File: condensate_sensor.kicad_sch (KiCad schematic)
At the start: 3 parts

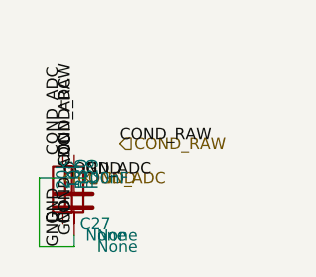
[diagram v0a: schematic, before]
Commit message: fic placer for small schemes
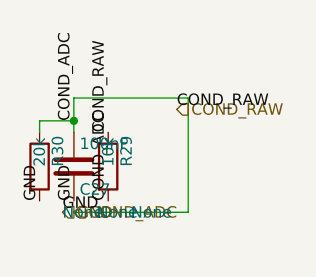
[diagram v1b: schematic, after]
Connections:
- net COND_ADC: no longer C27.2, R30.2
- new net GND: C27.2, R30.2
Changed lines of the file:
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@@
 	(symbol
 		(lib_id "Device:C")
-		(at 16.51 19.05 0)
+		(at 16.51 15.24 0)
 		(unit 1)
 		(exclude_from_sim no)
@@
 		(fields_autoplaced no)
 		(property "Reference" "C27"
-			(at 17.145 21.59 0.0000)
+			(at 17.145 17.78 0.0000)
 			(effects
 				(font
@@
 		)
 		(property "Value" "100nF"
-			(at 17.145 16.51 0.0000)
+			(at 17.145 12.7 0.0000)
 			(effects
 				(font
@@
 		)
 		(property "mirror" "None"
-			(at 19.05 24.1299 0)
+			(at 19.05 20.3199 0)
 			(effects
 				(font
@@
 		(instances
 			(project "Untitled"
-				(path "/aeae88a2-db2d-48e3-a72d-65ba09dff43f"
+				(path "/6ad2648c-8bf5-446b-ae62-81d18f8efea8"
 					(reference "C27")
 					(unit 1)
@@
 	(symbol
 		(lib_id "Device:R")
-		(at 16.51 17.78 0)
+		(at 20.32 15.24 0)
 		(unit 1)
 		(exclude_from_sim no)
@@
 		(fields_autoplaced no)
 		(property "Reference" "R29"
-			(at 18.542 17.78 90)
+			(at 22.352 15.24 90)
 			(effects
 				(font
@@
 		)
 		(property "Value" "10k"
-			(at 16.51 17.78 90)
+			(at 20.32 15.24 90)
 			(effects
 				(font
@@
 		)
 		(property "mirror" "None"
-			(at 19.05 22.8599 0)
+			(at 22.86 20.3199 0)
 			(effects
 				(font
@@
 		(instances
 			(project "Untitled"
-				(path "/aeae88a2-db2d-48e3-a72d-65ba09dff43f"
+				(path "/6ad2648c-8bf5-446b-ae62-81d18f8efea8"
 					(reference "R29")
 					(unit 1)
@@
 	(symbol
 		(lib_id "Device:R")
-		(at 15.24 17.78 0)
+		(at 12.7 15.24 0)
 		(unit 1)
 		(exclude_from_sim no)
@@
 		(fields_autoplaced no)
 		(property "Reference" "R30"
-			(at 17.272 17.78 90)
+			(at 14.732 15.24 90)
 			(effects
 				(font
@@
 		)
 		(property "Value" "20k"
-			(at 15.24 17.78 90)
+			(at 12.7 15.24 90)
 			(effects
 				(font
@@
 		)
 		(property "mirror" "None"
-			(at 17.78 22.8599 0)
+			(at 15.24 20.3199 0)
 			(effects
 				(font
@@
 		(instances
 			(project "Untitled"
-				(path "/aeae88a2-db2d-48e3-a72d-65ba09dff43f"
+				(path "/6ad2648c-8bf5-446b-ae62-81d18f8efea8"
 					(reference "R30")
 					(unit 1)
@@
 	(wire
 		(pts
-			(xy 16.51 22.86) (xy 16.51 24.13)
-		)
-		(stroke
-			(width 0)
-			(type default)
-		)
-	)
-	(wire
-		(pts
-			(xy 16.51 24.13) (xy 12.7 24.13)
-		)
-		(stroke
-			(width 0)
-			(type default)
-		)
-	)
-	(wire
-		(pts
-			(xy 12.7 24.13) (xy 12.7 16.51)
-		)
-		(stroke
-			(width 0)
-			(type default)
-		)
-	)
-	(wire
-		(pts
-			(xy 12.7 16.51) (xy 17.78 16.51)
-		)
-		(stroke
-			(width 0)
-			(type default)
-		)
+			(xy 12.7 11.43) (xy 12.7 10.16)
+		)
+		(stroke
+			(width 0)
+			(type default)
+		)
+	)
+	(wire
+		(pts
+			(xy 12.7 10.16) (xy 16.51 10.16)
+		)
+		(stroke
+			(width 0)
+			(type default)
+		)
+	)
+	(wire
+		(pts
+			(xy 16.51 10.16) (xy 16.51 11.43)
+		)
+		(stroke
+			(width 0)
+			(type default)
+		)
+	)
+	(wire
+		(pts
+			(xy 16.51 20.32) (xy 26.67 20.32)
+		)
+		(stroke
+			(width 0)
+			(type default)
+		)
+	)
+	(wire
+		(pts
+			(xy 26.67 20.32) (xy 29.21 20.32)
+		)
+		(stroke
+			(width 0)
+			(type default)
+		)
+	)
+	(wire
+		(pts
+			(xy 29.21 20.32) (xy 29.21 7.62)
+		)
+		(stroke
+			(width 0)
+			(type default)
+		)
+	)
+	(wire
+		(pts
+			(xy 29.21 7.62) (xy 16.51 7.62)
+		)
+		(stroke
+			(width 0)
+			(type default)
+		)
+	)
+	(wire
+		(pts
+			(xy 16.51 7.62) (xy 16.51 10.16)
+		)
+		(stroke
+			(width 0)
+			(type default)
+		)
+	)
+	(junction
+		(at 16.51 10.16)
+		(diameter 0)
+		(color 0 0 0 0)
 	)
 	(label "GND"
-		(at 15.24 21.59 270)
+		(at 16.51 19.05 270)
 		(effects
 			(font
@@
 	)
 	(label "GND"
-		(at 16.51 22.86 270)
+		(at 15.24 20.32 180)
 		(effects
 			(font
@@
 	)
 	(label "GND"
-		(at 17.78 16.51 180)
-		(effects
-			(font
-				(size 1.27 1.27)
-			)
-			(justify left bottom)
-		)
-	)
-	(label "GND"
-		(at 15.24 24.13 270)
+		(at 12.7 19.05 270)
 		(effects
 			(font
@@
 	)
 	(label "COND_RAW"
-		(at 16.51 13.97 90)
+		(at 20.32 11.43 90)
 		(effects
 			(font
@@
 	)
 	(label "COND_RAW"
-		(at 21.59 12.7 180)
+		(at 27.94 8.89 180)
 		(effects
 			(font
@@
 	)
 	(label "COND_ADC"
-		(at 15.24 13.97 90)
+		(at 20.32 19.05 270)
 		(effects
 			(font
@@
 	)
 	(label "COND_ADC"
-		(at 16.51 15.24 90)
-		(effects
-			(font
-				(size 1.27 1.27)
-			)
-			(justify left bottom)
-		)
-	)
-	(label "COND_ADC"
-		(at 15.24 16.51 0.0000)
-		(effects
-			(font
-				(size 1.27 1.27)
-			)
-			(justify left bottom)
-		)
-	)
-	(label "COND_ADC"
-		(at 16.51 21.59 270)
+		(at 16.51 10.16 270)
 		(effects
 			(font
@@
 	(hierarchical_label "GND"
 		(shape input)
-		(at 17.78 16.51 180)
+		(at 15.24 20.32 180)
 		(effects
 			(font
@@
 	(hierarchical_label "COND_RAW"
 		(shape input)
-		(at 21.59 12.7 180)
+		(at 27.94 8.89 180)
 		(effects
 			(font
@@
 	(hierarchical_label "COND_ADC"
 		(shape input)
-		(at 15.24 16.51 0)
-		(effects
-			(font
+		(at 16.51 20.32 0)
+		(effects
+			(font
